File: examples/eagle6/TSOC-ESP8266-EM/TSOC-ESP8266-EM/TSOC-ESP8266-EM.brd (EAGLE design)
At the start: 38.4 x 26.4 mm, 33 parts, among them Q1 MMBT2222A, U1 ESP8266-12-12W, U2 EEPROM-I2CSMD, U3 TMP102, U4 ATECC108

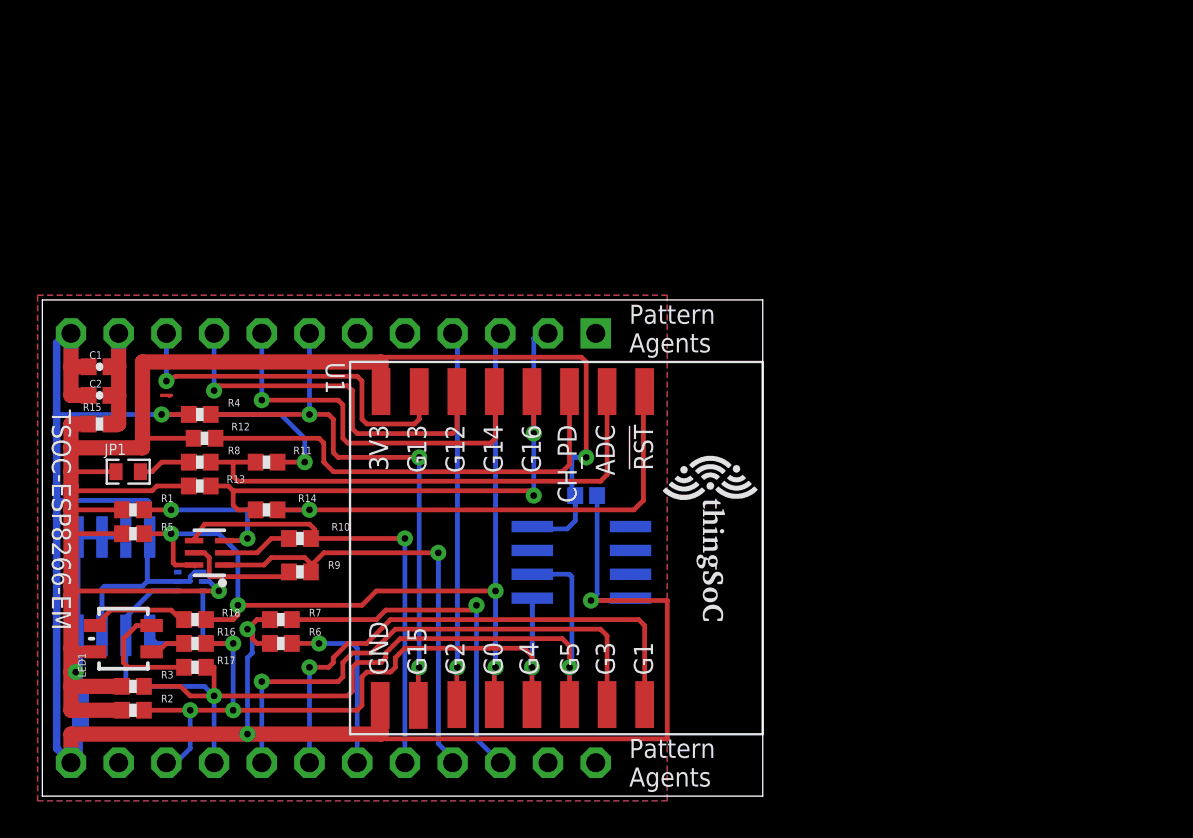
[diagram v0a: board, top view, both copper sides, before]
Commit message: update modules
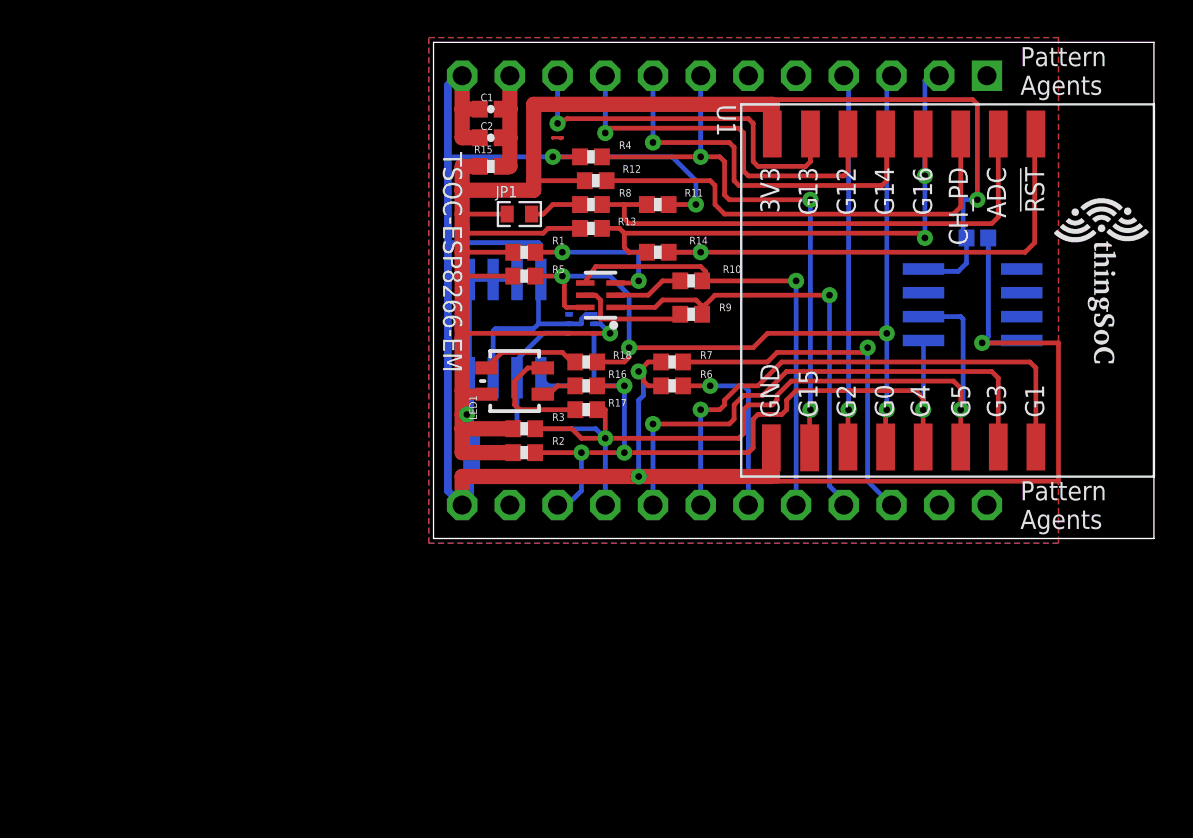
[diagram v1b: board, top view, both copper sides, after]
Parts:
- moved C3 24.9 mm to (2.29, 5.08)
- moved C4 24.9 mm to (29.2, 16.5)
- moved R12 24.9 mm to (8.89, 19.6)
- moved U1 24.9 mm to (27.2, 13.5)
- moved C1 24.9 mm to (3.30, 23.4)
- moved C2 24.9 mm to (3.30, 21.8)
- moved JP1 24.9 mm to (4.83, 17.8)
- moved LED1 24.9 mm to (4.57, 8.89)
- moved Q1 24.9 mm to (9.14, 13.5)
- moved R1 24.9 mm to (5.08, 15.7)
- moved R10 24.9 mm to (14.0, 14.2)
- moved R11 24.9 mm to (12.2, 18.3)
- moved R13 24.9 mm to (8.64, 17.0)
- moved R14 24.9 mm to (12.2, 15.7)
- moved R15 24.9 mm to (3.30, 20.3)
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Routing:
- net GND: track 131.7 -> 132.4 mm
